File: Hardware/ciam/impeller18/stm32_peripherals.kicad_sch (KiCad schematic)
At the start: 8 parts, among them J1 Micro_SD_Card_Con

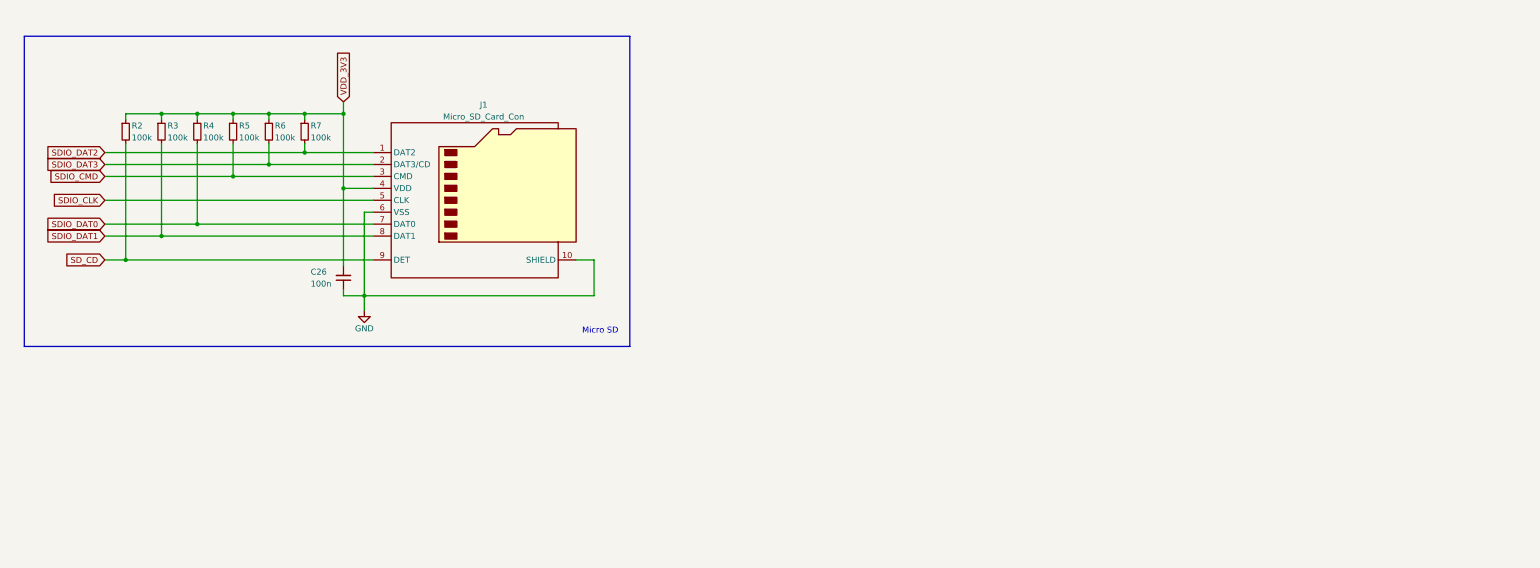
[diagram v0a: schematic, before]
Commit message: updated impeller18 schematics
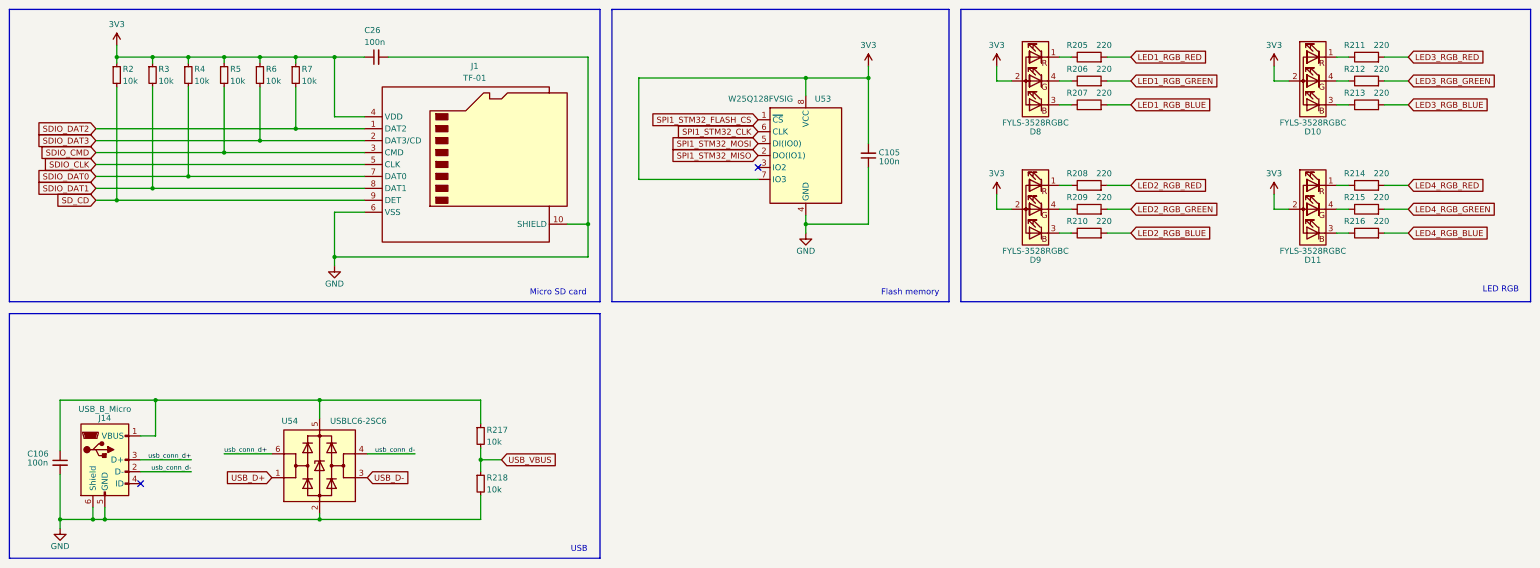
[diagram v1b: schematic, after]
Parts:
- added C105, C106: 100n, Capacitor_SMD:C_0603_1608Metric, symbol Device:C_Small
- added D10, D11, D8, D9: FYLS-3528RGBC, user_lib:LED_RGB_promelec, symbol Device:LED_RGBA
- added J14: USB_B_Micro, user_lib:U-F-M5DD-W-2-SUS, symbol Connector:USB_B_Micro
- added R205, R206, R207, R208, R209, R210, R211, R212, R213, R214, R215, R216: 220, Resistor_SMD:R_0603_1608Metric, symbol Device:R
- added R217, R218: 10k, Resistor_SMD:R_0603_1608Metric, symbol Device:R_Small
- added U53: W25Q128FVSIG, Package_SO:SOIC-8_5.23x5.23mm_P1.27mm, symbol Memory_Flash:W25Q32JVSS
- added U54: USBLC6-2SC6, Package_TO_SOT_SMD:SOT-23-6, symbol Power_Protection:USBLC6-2SC6
- J1: value Micro_SD_Card_Con -> TF-01
- R2, R3, R4, R5, R6, R7: value 100k -> 10k
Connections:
- net GND: now also C26.2, C105.1, C106.2, J14.5 (GND), J14.6 (Shield), R218.2, U53.4 (GND), U54.2 (GND); no longer C26.1
- net VDD_3V3 renamed 3V3
- net 3V3: now also C26.1, C105.2, D10.2 (A), D11.2 (A), D8.2 (A), D9.2 (A), U53.7 (IO3), U53.8 (VCC); no longer C26.2
- new net: D8.3 (BK), R207.1
- new net: D9.1 (RK), R208.1
- new net: D9.4 (GK), R209.1
- new net: D8.4 (GK), R206.1
- new net: D10.3 (BK), R213.1
- new net: D11.4 (GK), R215.1
- new net: D11.1 (RK), R214.1
- new net: C106.1, J14.1 (VBUS), R217.1, U54.5 (VBUS)
- new net: D9.3 (BK), R210.1
- new net: D8.1 (RK), R205.1
- new net: D10.1 (RK), R211.1
- new net: D10.4 (GK), R212.1
- new net: D11.3 (BK), R216.1
- new net LED1_RGB_BLUE: R207.2
- new net LED1_RGB_GREEN: R206.2
- new net LED1_RGB_RED: R205.2
- new net LED2_RGB_BLUE: R210.2
- new net LED2_RGB_GREEN: R209.2
- new net LED2_RGB_RED: R208.2
- new net LED3_RGB_BLUE: R213.2
- new net LED3_RGB_GREEN: R212.2
- new net LED3_RGB_RED: R211.2
- new net LED4_RGB_BLUE: R216.2
- new net LED4_RGB_GREEN: R215.2
- new net LED4_RGB_RED: R214.2
- new net SPI1_STM32_CLK: U53.6 (CLK)
- new net SPI1_STM32_FLASH_CS: U53.1 (~{CS})
- new net SPI1_STM32_MISO: U53.2 (DO(IO1))
- new net SPI1_STM32_MOSI: U53.5 (DI(IO0))
- new net USB_D+: U54.1 (I/O1)
- new net USB_D-: U54.3 (I/O2)
- new net USB_VBUS: R217.2, R218.1
- new net usb_conn_d+: J14.3 (D+), U54.6 (I/O1)
- new net usb_conn_d-: J14.2 (D-), U54.4 (I/O2)
- no-connect marks 0 -> 2
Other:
- note added: "Flash memory"
- note added: "LED RGB"
- note added: "Micro SD card"
- note added: "USB"
- note removed: "Micro SD"
- moved on the sheet: R2
